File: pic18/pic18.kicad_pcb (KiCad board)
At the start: 2 copper layers, 90.2 x 99.1 mm, 104 parts, among them J1 PORTA, J10 PORTD, J11 PORTD1, J12 PORTC, J13 PORTC1, J14 PICKIT3, J15 CONTROL, J16 5V, J17 3.3V, J18 5V, J19 3.3V, J2 PORTB, J20 LED'S, J21 BUZZER, J22 PORTE, J23 PORTE1, J4 Barrel_Jack_Switch, J5 TECLADO, J6 Conn_01x04, J7 PORTA1, J8 HC-05, J9 PORTB1, Q1 2N3906, Q2 2N2219, Q3 2N2219, Q4 2N2219, SW1 SW_Push, SW2 SW_DIP_x01, U1 PIC18F45K50, U2 3x7Segment, U3 NRF24L01_Breakout

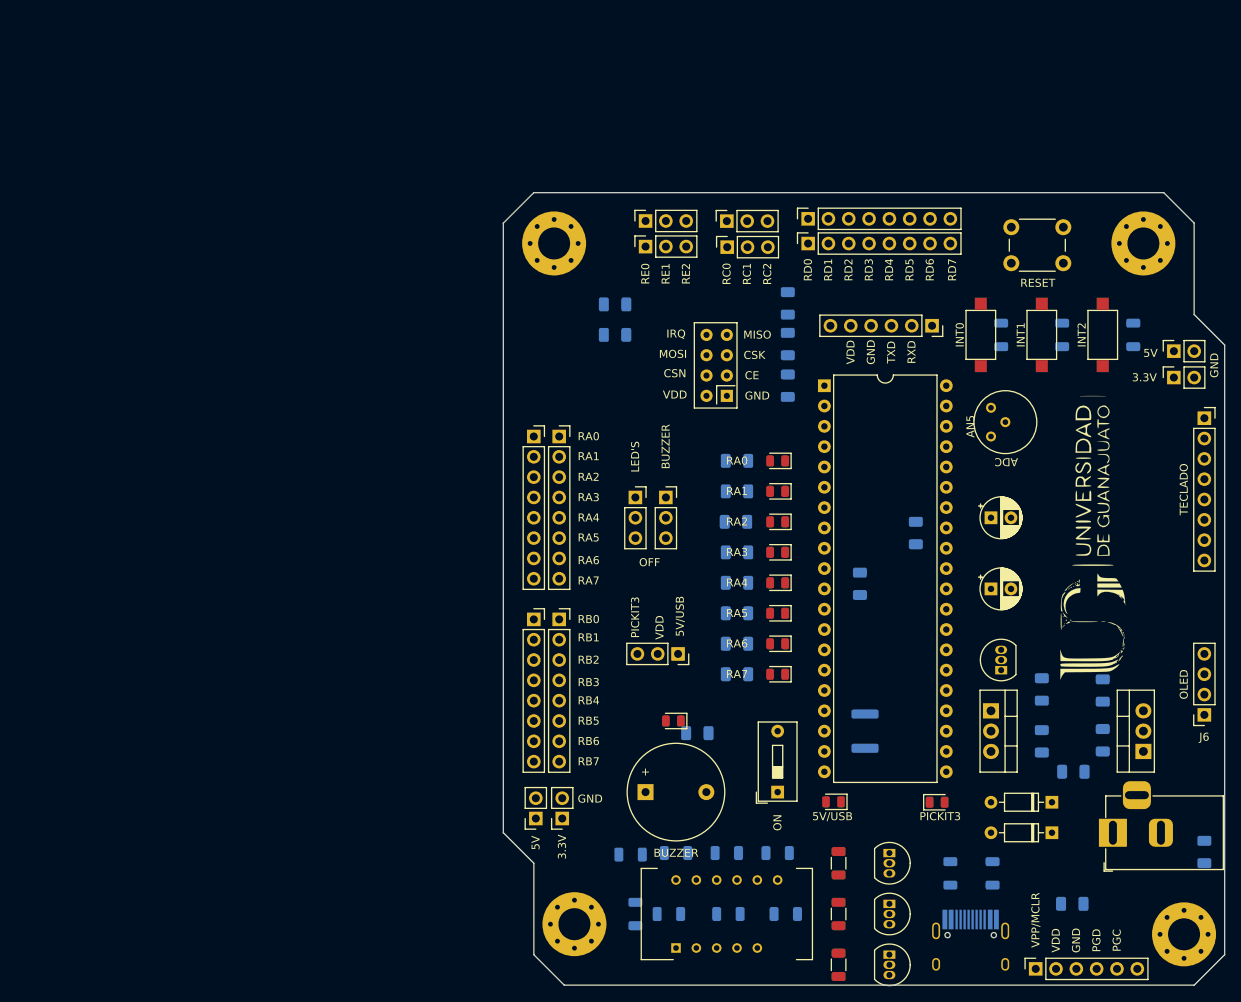
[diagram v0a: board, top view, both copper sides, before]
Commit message: JaPic
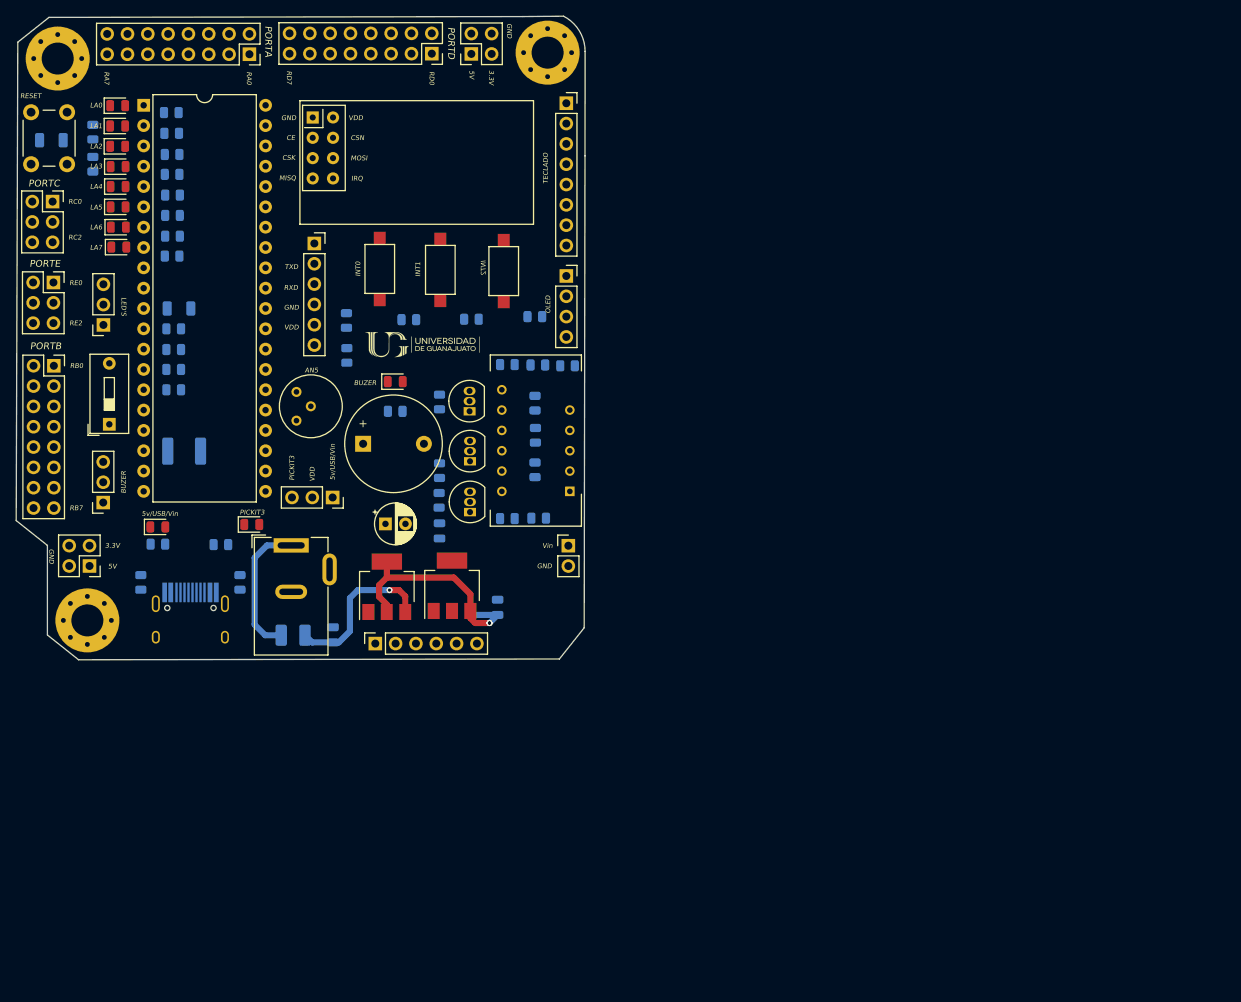
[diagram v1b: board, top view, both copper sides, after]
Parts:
- removed 3.3v1, 5v1: L7805, Package_TO_SOT_THT:TO-220-3_Vertical
- removed C6: 0.33uf, Capacitor_THT:CP_Radial_D5.0mm_P2.50mm
- removed C7: 100nf, Capacitor_SMD:C_1206_3216Metric
- removed D2: 1N4148, Diode_THT:D_DO-35_SOD27_P7.62mm_Horizontal
- removed D3: LED, LED_SMD:LED_0805_2012Metric
- removed the G*** at (173.6, 82.4)
- removed the G*** at (106.7, 61.0)
- removed the G*** at (101.5, 65.7)
- removed the G*** at (101.2, 57.2)
- removed the G*** at (171.4, 85.1)
- removed H4: MountingHole, MountingHole:MountingHole_4mm_Pad_Via
- removed J13: PORTC1, Connector_PinSocket_2.54mm:PinSocket_1x03_P2.54mm_Vertical
- removed J16, J18: 5V, Connector_PinSocket_2.54mm:PinSocket_1x02_P2.54mm_Vertical
- removed J17, J19: 3.3V, Connector_PinSocket_2.54mm:PinSocket_1x02_P2.54mm_Vertical
- removed J22: PORTE, Connector_PinSocket_2.54mm:PinSocket_1x03_P2.54mm_Vertical
- removed J23: PORTE1, Connector_PinSocket_2.54mm:PinSocket_1x03_P2.54mm_Vertical
- removed Q1: 2N3906, Package_TO_SOT_THT:TO-92_Inline
- removed Q2, Q3, Q4: 2N2219, Package_TO_SOT_THT:TO-92_Inline
- added C9: 0.1uF, Capacitor_SMD:C_0805_2012Metric, B.Cu at (76.5, 97.2)
- added D14: 1N4007, Diode_SMD:D_1210_3225Metric_Pad1.42x2.65mm_HandSolder, B.Cu at (71.5, 97.2)
- added DIG1: 2N2219, Package_TO_SOT_THT:TO-92_Inline, F.Cu at (93.6, 81.8)
- added DIG2: 2N2219, Package_TO_SOT_THT:TO-92_Inline, F.Cu at (93.6, 75.5)
- added DIG3: 2N2219, Package_TO_SOT_THT:TO-92_Inline, F.Cu at (93.6, 69.2)
- added G1: LOGO, FIMEE:japic, B.Cu at (89.8, 41.7)
- added G2: LOGO, FIMEE:kicad_logo, B.Cu at (99.8, 34.5)
- added G3: LOGO, FIMEE:open_hardware, B.Cu at (99.3, 41.9)
- added G4: LOGO, FIMEE:github, B.Cu at (98.8, 48.8)
- added G5: LOGO, FIMEE:fimee, F.Cu at (87.7, 60.8)
- added G6: LOGO, FIMEE:abeja_sf, F.Cu at (91.2, 37.8)
- added J3: Barrel_Jack_Switch, Connector_BarrelJack:BarrelJack_Wuerth_6941xx301002, F.Cu at (71.3, 86.0)
- added R34: 470, Resistor_SMD:R_0805_2012Metric, B.Cu at (54.6, 85.9)
- added U4: AMS1117-5.0, Package_TO_SOT_SMD:SOT-223-3_TabPin2, F.Cu at (83.2, 91.2)
- added U5: AMS1117-3.3, Package_TO_SOT_SMD:SOT-223-3_TabPin2, F.Cu at (91.4, 91.0)
- C3: value 100nf -> 100uF; footprint Capacitor_SMD:C_1206_3216Metric -> Capacitor_THT:CP_Radial_D5.0mm_P2.50mm; moved to F.Cu
- C4: value 220uf -> 0.1uF; footprint Capacitor_THT:CP_Radial_D5.0mm_P2.50mm -> Capacitor_SMD:C_0805_2012Metric; moved to B.Cu
- C5: value 100nf -> 0.1uF; footprint Capacitor_SMD:C_1206_3216Metric -> Capacitor_SMD:C_0805_2012Metric
- D1: value 1N4148 -> LED; footprint Diode_THT:D_DO-35_SOD27_P7.62mm_Horizontal -> LED_SMD:LED_0805_2012Metric
- D10: value LED -> LED10
- D11, D5: value LED -> LED11
- D4: value LED -> LED4
- D6: value LED -> LED6
- D7: value LED -> LED7
- D8: value LED -> LED8
- D9: value LED -> LED9
- H1: value MountingHole -> 1
- H2: value MountingHole -> 2
- H3: value MountingHole -> 3
- J1, J2: footprint Connector_PinSocket_2.54mm:PinSocket_1x08_P2.54mm_Vertical -> Connector_PinSocket_2.54mm:PinSocket_2x08_P2.54mm_Vertical
- J10: value PORTD -> PORTE; footprint Connector_PinSocket_2.54mm:PinSocket_1x08_P2.54mm_Vertical -> Connector_PinSocket_2.54mm:PinSocket_2x03_P2.54mm_Vertical
- J11: value PORTD1 -> 5v-3.3v; footprint Connector_PinSocket_2.54mm:PinSocket_1x08_P2.54mm_Vertical -> Connector_PinSocket_2.54mm:PinSocket_2x02_P2.54mm_Vertical
- J12: value PORTC -> 5v-3.3v; footprint Connector_PinSocket_2.54mm:PinSocket_1x03_P2.54mm_Vertical -> Connector_PinSocket_2.54mm:PinSocket_2x02_P2.54mm_Vertical
- J4: value Barrel_Jack_Switch -> Vin; footprint Connector_BarrelJack:BarrelJack_Horizontal -> Connector_PinHeader_2.54mm:PinHeader_1x02_P2.54mm_Vertical
- J6: value Conn_01x04 -> OLED
- J7: value PORTA1 -> PORTD; footprint Connector_PinSocket_2.54mm:PinSocket_1x08_P2.54mm_Vertical -> Connector_PinSocket_2.54mm:PinSocket_2x08_P2.54mm_Vertical
- J9: value PORTB1 -> PORTC; footprint Connector_PinSocket_2.54mm:PinSocket_1x08_P2.54mm_Vertical -> Connector_PinSocket_2.54mm:PinSocket_2x03_P2.54mm_Vertical
- R1, R10, R11, R12, R13, R14, R15, R16, R17, R18, R19, R20, R21, R22, R23, R25, R26, R27, R28, R29, R30, R31, R32, R6, R7, R8, R9: footprint Resistor_SMD:R_1206_3216Metric -> Resistor_SMD:R_0805_2012Metric
- R2, R3: value 5.6k -> 4.7; footprint Resistor_SMD:R_1206_3216Metric -> Resistor_SMD:R_0805_2012Metric
- R24, R33, R37: footprint Resistor_SMD:R_1206_3216Metric -> Resistor_SMD:R_0805_2012Metric; moved to B.Cu
- R4: value 10k -> 4.7; footprint Resistor_SMD:R_1206_3216Metric -> Resistor_SMD:R_0805_2012Metric
- R5: value 470 -> 4.7; footprint Resistor_SMD:R_1206_3216Metric -> Resistor_SMD:R_0805_2012Metric
- moved R2 141.2 mm to (56.6, 66.5), turned to 0 degrees
- moved H3 140.2 mm to (45.8, 95.4)
- moved R3 125.0 mm to (56.6, 64.0), turned to 0 degrees
- moved R4 123.7 mm to (56.6, 61.5), turned to 180 degrees
- moved SW1 122.8 mm to (38.8, 38.4), turned to 90 degrees
- moved D1 118.1 mm to (54.6, 83.7), turned to 0 degrees
- moved R5 117.5 mm to (56.6, 58.9), turned to 0 degrees
- moved R22 115.5 mm to (62.5, 85.9)
- moved H2 109.0 mm to (103.3, 24.4)
- moved R1 107.5 mm to (52.5, 90.6)
- moved USB1 105.8 mm to (58.7, 100.1)
- moved G*** 105.4 mm to (58.9, 94.7)
- moved R10 100.9 mm to (64.9, 90.6), turned to 90 degrees
- moved J11 98.5 mm to (46.1, 88.6), turned to 270 degrees
- moved D4 98.1 mm to (49.7, 48.7), turned to 0 degrees
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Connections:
- C1 pad 1: VDD -> Net-(C1-Pad1)
- C3 pad 1: Net-(5v1-Pad3) -> Net-(C3-Pad1)
- C4 pad 1: GND -> Net-(C3-Pad1)
- C4 pad 2: 5V -> GND
- C5 pad 1: VDD -> 3.3v
- D1 pad 1: GND -> Net-(D1-Pad1)
- D1 pad 2: Net-(5v1-Pad2) -> Net-(C3-Pad1)
- H1 pad 1: (no net) -> GND
- H2 pad 1: (no net) -> GND
- H3 pad 1: (no net) -> GND
- J1 pad 2: /RA1 -> /RA0
- J1 pad 3: /RA2 -> /RA1
- J1 pad 4: /RA3 -> /RA1
- J1 pad 5: /RA4 -> /RA2
- J1 pad 6: /RA5 -> /RA2
- J1 pad 7: /RA6 -> /RA3
- J1 pad 8: /RA7 -> /RA3
- J10 pad 1: /RD0 -> /RE0
- J10 pad 2: /RD1 -> /RE0
- J10 pad 3: /RD2 -> /RE1
- J10 pad 4: /RD3 -> /RE1
- J10 pad 5: /RD4 -> /RE2
- J10 pad 6: /RD5 -> /RE2
- J11 pad 1: /RD0 -> VDD
- J11 pad 2: /RD1 -> 3.3v
- J11 pad 3: /RD2 -> GND
- J11 pad 4: /RD3 -> GND
- J12 pad 1: /RC0 -> VDD
- J12 pad 2: /RC1 -> 3.3v
- J12 pad 3: /RC2 -> GND
- J2 pad 2: /RB1 -> /RB0
- J2 pad 3: /RB2 -> /RB1
- J2 pad 4: /RB3 -> /RB1
- J2 pad 5: /RB4 -> /RB2
- J2 pad 6: /RB5 -> /RB2
- J2 pad 7: /RB6 -> /RB3
- J2 pad 8: /RB7 -> /RB3
- J4 pad 1: Net-(5v1-Pad1) -> /Vin
- J7 pad 1: /RA0 -> /RD0
- J7 pad 2: /RA1 -> /RD0
- J7 pad 3: /RA2 -> /RD1
- J7 pad 4: /RA3 -> /RD1
- J7 pad 5: /RA4 -> /RD2
- J7 pad 6: /RA5 -> /RD2
- J7 pad 7: /RA6 -> /RD3
- J7 pad 8: /RA7 -> /RD3
- J9 pad 1: /RB0 -> /RC0
- J9 pad 2: /RB1 -> /RC0
- J9 pad 3: /RB2 -> /RC1
- J9 pad 4: /RB3 -> /RC1
- J9 pad 5: /RB4 -> /RC2
- J9 pad 6: /RB5 -> /RC2
- R2 pad 1: Net-(5v1-Pad3) -> VDD
- R2 pad 2: GND -> Net-(R2-Pad2)
- R25 pad 2: /RB6 -> /RD6
- R26 pad 2: /RB5 -> /RD5
- R27 pad 2: /RB4 -> /RD4
- R28 pad 2: /RB3 -> /RD3
- R29 pad 2: /RB2 -> /RD2
- R3 pad 1: Net-(Q1-Pad2) -> Net-(R2-Pad2)
- R3 pad 2: Net-(5v1-Pad3) -> Net-(R3-Pad2)
- R30 pad 2: /RB1 -> /RD1
- R31 pad 2: /RB0 -> /RD0
- R32 pad 2: /RB7 -> /RD7
- R4 pad 1: /VUSB -> Net-(R3-Pad2)
- R4 pad 2: GND -> Net-(R4-Pad2)
- R5 pad 1: Net-(D3-Pad2) -> Net-(R4-Pad2)
- R5 pad 2: 5V -> Net-(C1-Pad1)
- U1 pad 11: VDD -> Net-(C1-Pad1)
- U1 pad 32: VDD -> Net-(U1-Pad32)
- USB1 pad 11: /VUSB -> 5V
- USB1 pad 2: /VUSB -> 5V
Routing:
- net Net-(C3-Pad1): track 0.00 -> 28.5 mm, vias 0 -> 2
- net Net-(C9-Pad1): track 0.00 -> 20.3 mm, vias 0 -> 1
- net /Vin: track 0.00 -> 17.5 mm
- net GND: track 0.00 -> 1.62 mm
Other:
- board size 90.2 x 99.1 mm -> 71.1 x 80.4 mm
- board text added: "5v/USB/Vin"
- board text added: "@javimenba"
- board text added: "BUZER"
- board text added: "INT0"
- board text added: "INT1"
- board text added: "INT2"
- board text added: "LA0"
- board text added: "LA1"
- board text added: "LA2"
- board text added: "LA3"
- board text added: "LA4"
- board text added: "LA5"
- board text added: "LA6"
- board text added: "LA7"
- board text added: "MISQ"
- board text added: "PORTA"
- board text added: "PORTB"
- board text added: "PORTC"
- board text added: "PORTD"
- board text added: "PORTE"
- board text added: "Vin"
- board text removed: "2.5"
- board text removed: "5V/USB"
- board text removed: "ADC"
- board text removed: "BUZZER"
- board text removed: "MISO"
- board text removed: "OFF"
- board text removed: "ON"
- board text removed: "RA1"
- board text removed: "RA2"
- board text removed: "RA3"
- board text removed: "RA4"
- board text removed: "RA5"
- board text removed: "RA6"
- board text removed: "RB1"
- board text removed: "RB2"
- board text removed: "RB3"
- board text removed: "RB4"
- board text removed: "RB5"
- board text removed: "RB6"
- board text removed: "RC1"
- board text removed: "RD1"
- board text removed: "RD2"
- board text removed: "RD3"
- board text removed: "RD4"
- board text removed: "RD5"
- board text removed: "RD6"
- board text removed: "RE1"
